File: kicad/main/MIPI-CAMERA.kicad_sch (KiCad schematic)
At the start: 11 parts

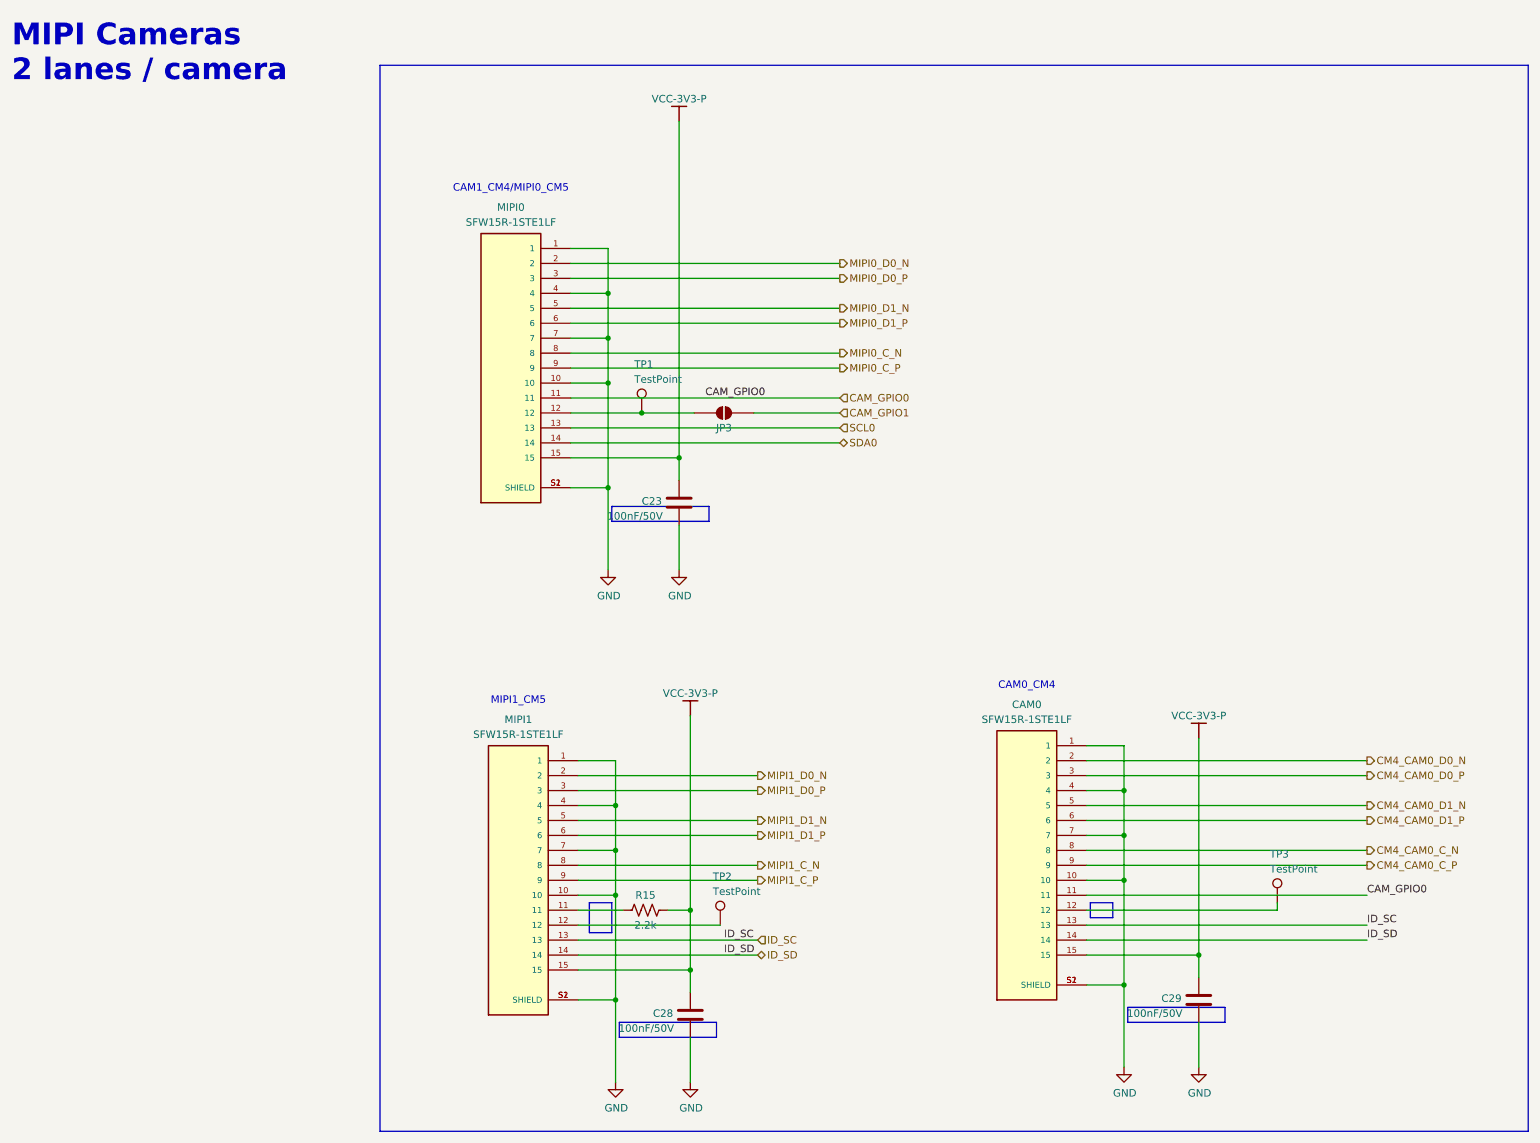
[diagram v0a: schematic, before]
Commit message: Second review round
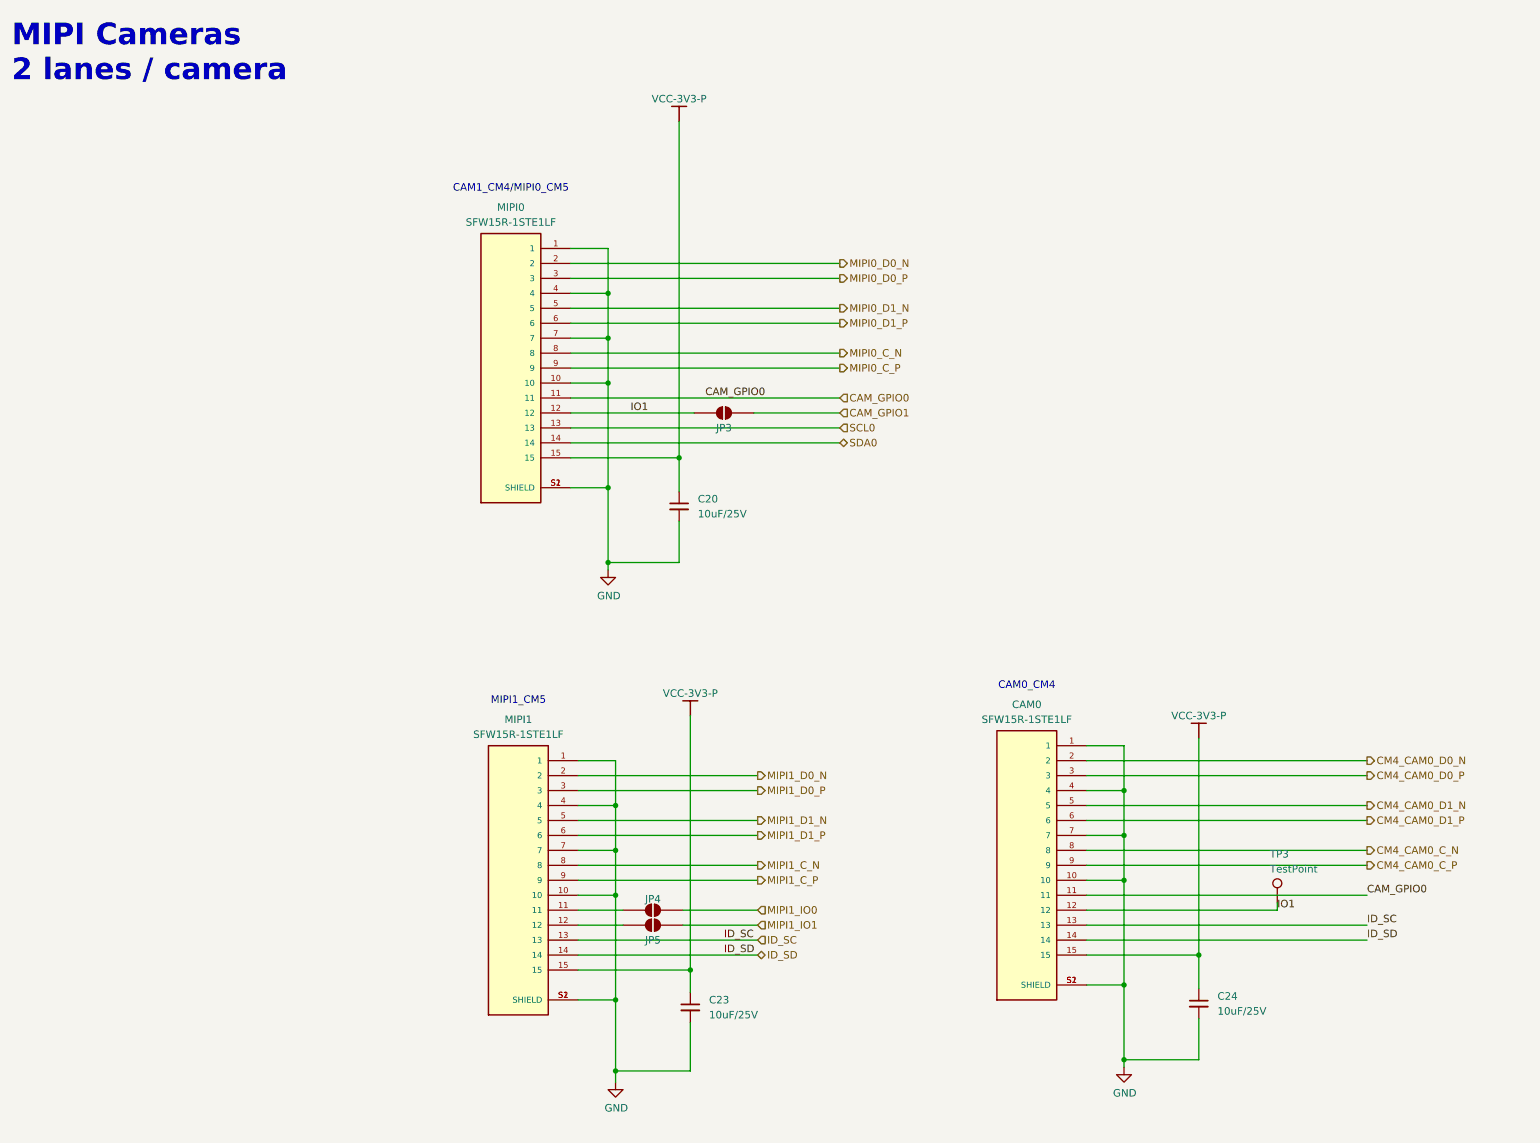
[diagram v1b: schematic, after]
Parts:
- removed C23, C28, C29: 100nF/50V, Capacitor_SMD:C_0603_1608Metric, symbol Device:C
- removed R15: 2.2k, Resistor_SMD:R_0603_1608Metric, symbol Device:R_US
- removed TP1, TP2: TestPoint, TestPoint:TestPoint_Pad_D2.0mm, symbol Connector:TestPoint
- added C20, C23, C24: 10uF/25V, Capacitor_SMD:C_0603_1608Metric, symbol Device:C_Small
- added JP4, JP5: (no value), Jumper:SolderJumper-2_P1.3mm_Open_RoundedPad1.0x1.5mm, symbol Jumper:SolderJumper_2_Open
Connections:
- net GND: now also C20.2, C23.2, C24.2
- net VCC-3V3-P: now also C20.1, C23.1, C24.1
- net IO1: now reaches JP3.1 (A), MIPI0.12
- net IO1: now also CAM0.12, TP3.1
- net at MIPI1.12: now also JP5.1 (A)
- net at MIPI1.11: now also JP4.1 (A)
- new net MIPI1_IO0: JP4.2 (B)
- new net MIPI1_IO1: JP5.2 (B)
